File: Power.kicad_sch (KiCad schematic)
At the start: 7 parts, among them J2 USB_C_Receptacle, U3 CP2102N-Axx-xQFN28

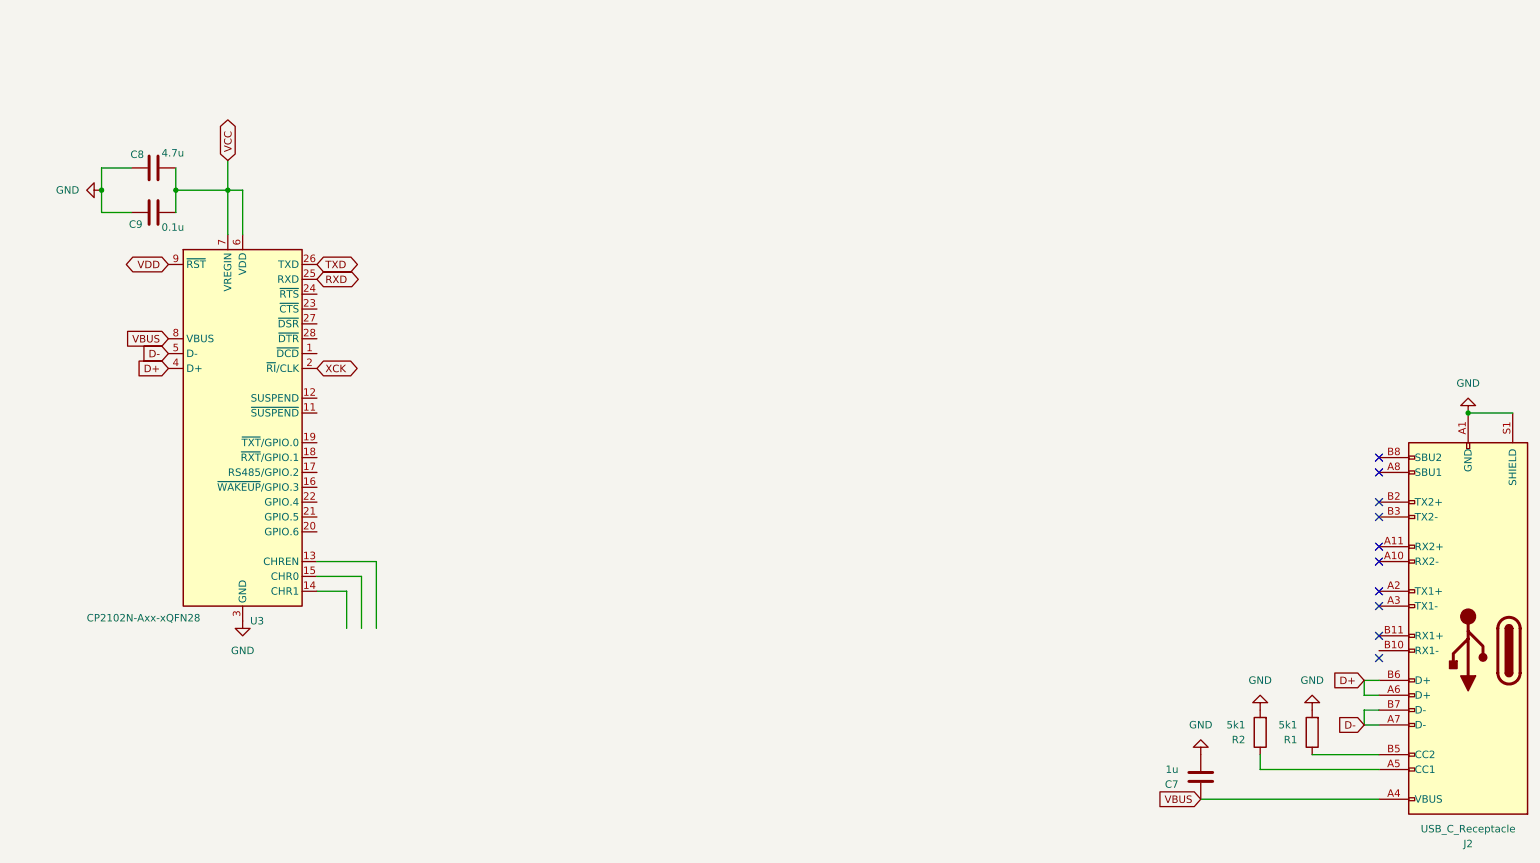
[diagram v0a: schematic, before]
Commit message: Draw basic inital schematic
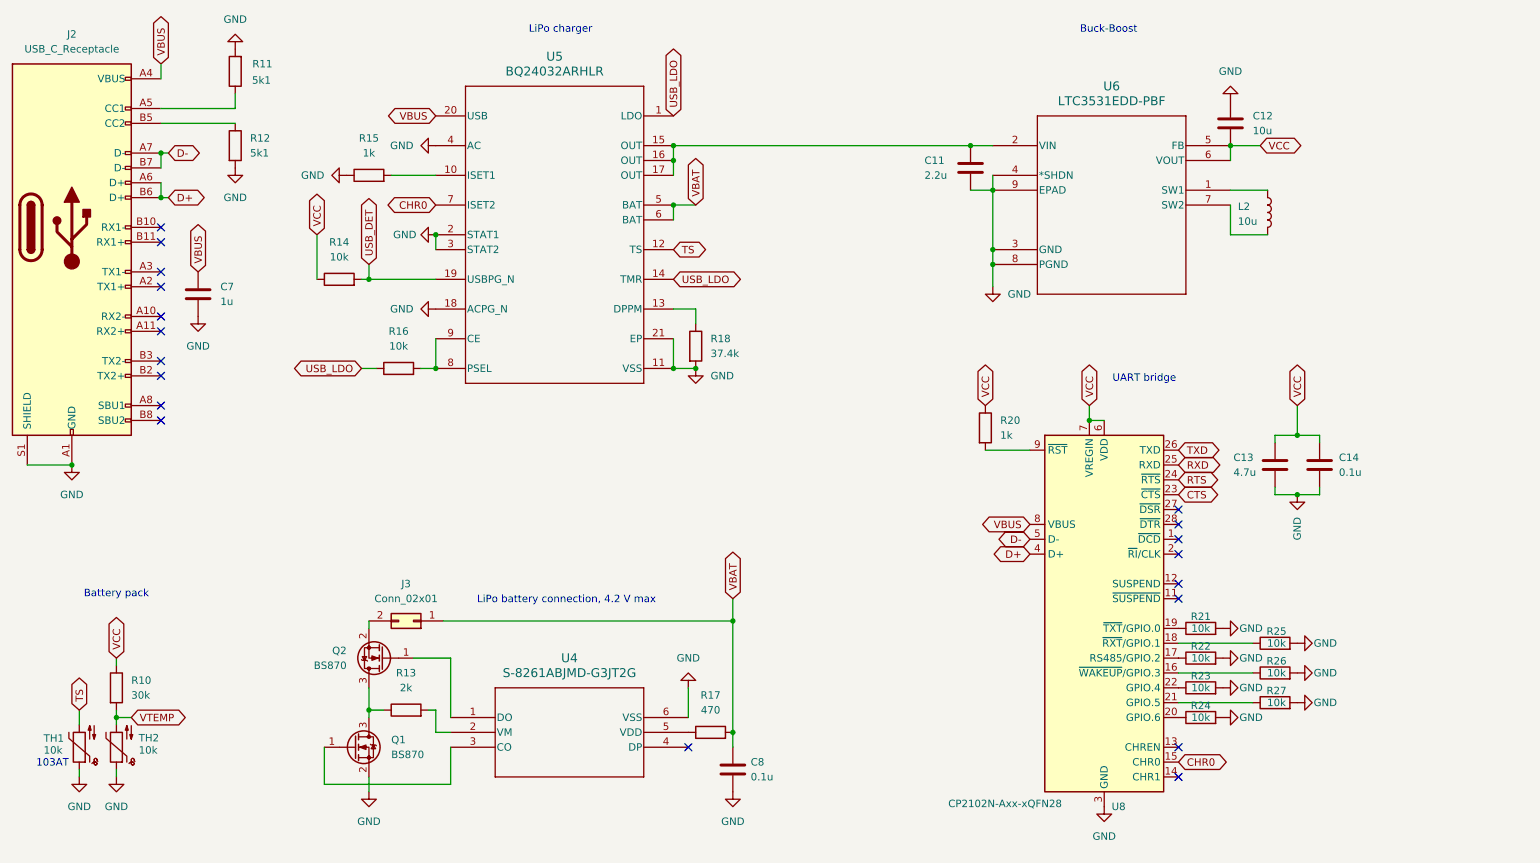
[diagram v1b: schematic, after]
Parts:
- removed C9: 0.1u, symbol Device:C
- added C11: 2.2u, symbol Device:C
- added C12: 10u, symbol Device:C
- added C13: 4.7u, symbol Device:C
- added C14: 0.1u, symbol Device:C
- added J3: Conn_02x01, symbol Connector_Generic:Conn_02x01
- added L2: 10u, symbol Device:L
- added Q1, Q2: BS870, Package_TO_SOT_SMD:SOT-23, symbol Transistor_FET:BS870
- added R10: 30k, symbol Device:R
- added R13: 2k, symbol Device:R
- added R14, R16, R21, R22, R23, R24, R25, R26, R27: 10k, symbol Device:R
- added R15, R20: 1k, symbol Device:R
- added R17: 470, symbol Device:R
- added R18: 37.4k, symbol Device:R
- added TH1, TH2: 10k, symbol Device:Thermistor_NTC
- added U4: S-8261ABJMD-G3JT2G, IC6_S-8261ABJMD-G3JT2G_ABL, symbol 2024-11-21_09-28-04:S-8261ABJMD-G3JT2G
- added U5: BQ24032ARHLR, RHL0020A, symbol 2024-11-20_19-55-08:BQ24032ARHLR
- added U6: LTC3531EDD-PBF, DFN-8_DD_LIT, symbol 2024-11-21_16-20-21:LTC3531EDD-PBF
- C8: value 4.7u -> 0.1u
- renumbered R2 to R11, R1 to R12, U3 to U8
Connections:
- net GND: now also C8.2, C11.2, C12.1, C13.2, C14.2, Q1.2 (S), R15.1, R18.2, R21.2, R22.2, R23.2, R24.2, R25.2, R26.2, R27.2, TH1.1, TH2.1, U4.6 (VSS), U5.11 (VSS), U5.18 (ACPG_N), U5.2 (STAT1), U5.21 (EP), U5.3 (STAT2), U5.4 (AC), U6.3 (GND), U6.4 (*SHDN), U6.8 (PGND), U6.9 (EPAD); no longer C8.1
- net VBUS: now also U5.20 (USB)
- net VCC: now also C12.2, C13.1, C14.1, R10.1, R14.1, R20.1, U6.5 (FB), U6.6 (VOUT); no longer C8.2
- net CHR0: now reaches U8.15 (CHR0)
- net CHR0: now also U5.7 (ISET2)
- net at U8.16 (~{WAKEUP}/GPIO.3): now also R26.1
- net at U8.17 (RS485/GPIO.2): now also R22.1
- net at U8.18 (~{RXT}/GPIO.1): now also R25.1
- net at U8.19 (~{TXT}/GPIO.0): now also R21.1
- net at U8.20 (GPIO.6): now also R24.1
- net at U8.21 (GPIO.5): now also R27.1
- net at U8.22 (GPIO.4): now also R23.1
- net CTS: now reaches U8.23 (~{CTS})
- net RTS: now reaches U8.24 (~{RTS})
- net VDD: no longer names the net of U8.9 (~{RST})
- net VDD: now also R20.2
- net XCK: no longer names the net of U8.2 (~{RI}/CLK)
- new net: Q1.1 (G), U4.3 (CO)
- new net: Q1.3 (D), Q2.3 (D), R13.1
- new net: L2.1, U6.1 (SW1)
- new net: C11.1, U5.15 (OUT), U5.16 (OUT), U5.17 (OUT), U6.2 (VIN)
- new net: L2.2, U6.7 (SW2)
- new net: Q2.1 (G), U4.1 (DO)
- new net: R13.2, U4.2 (VM)
- new net: R17.1, U4.5 (VDD)
- new net: J3.2 (Pin_2), Q2.2 (S)
- new net: R16.2, U5.8 (PSEL), U5.9 (CE)
- new net: R18.1, U5.13 (DPPM)
- new net: R15.2, U5.10 (ISET1)
- new net TS: TH1.2, U5.12 (TS)
- new net USB_DET: R14.2, U5.19 (USBPG_N)
- new net USB_LDO: R16.1, U5.1 (LDO), U5.14 (TMR)
- new net VBAT: C8.1, J3.1 (Pin_1), R17.2, U5.5 (BAT), U5.6 (BAT)
- new net VTEMP: R10.2, TH2.2
- no-connect marks 10 -> 19
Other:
- note added: "103AT"
- note added: "Battery pack"
- note added: "Buck-Boost"
- note added: "LiPo battery connection, 4.2 V max"
- note added: "LiPo charger"
- note added: "UART bridge"
- moved on the sheet: C7, J2, R11, R12, U8
